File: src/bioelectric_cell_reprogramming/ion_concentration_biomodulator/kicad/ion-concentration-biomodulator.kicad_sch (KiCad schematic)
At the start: 43 parts, among them J1 532610671, J10 39-53-2045, J11 Conn_01x14_Pin, J12 Conn_01x14_Pin, J13 39-53-2045, J14 39-53-2045, J15 Conn_ARM_SWD_TagConnect_TC2030, J16 IPL1-104-01-L-D-K, J17 Conn_01x02_Pin, J18 EJ508A, J19 USB_C_Receptacle_USB2.0_14P, J2 532610671, J21 IPL1-102-01-L-S-K, J22 IPL1-104-01-X-S-K, J3 532610671, J4 532610671, J5 S4B-PH-SM4-TB, J6 Conn_01x02_Pin, J8 39-53-2045, J9 IPL1-102-01-L-S-K, Q1 NDT3055L, Q2 NDT3055L, Q4 NDT3055L, Q5 NDT3055L, Q6 NDT3055L, SW1 SW_Push, U2 LM1084-5.0, U3 LM1084-3.3, U4 USBLC6-2SC6

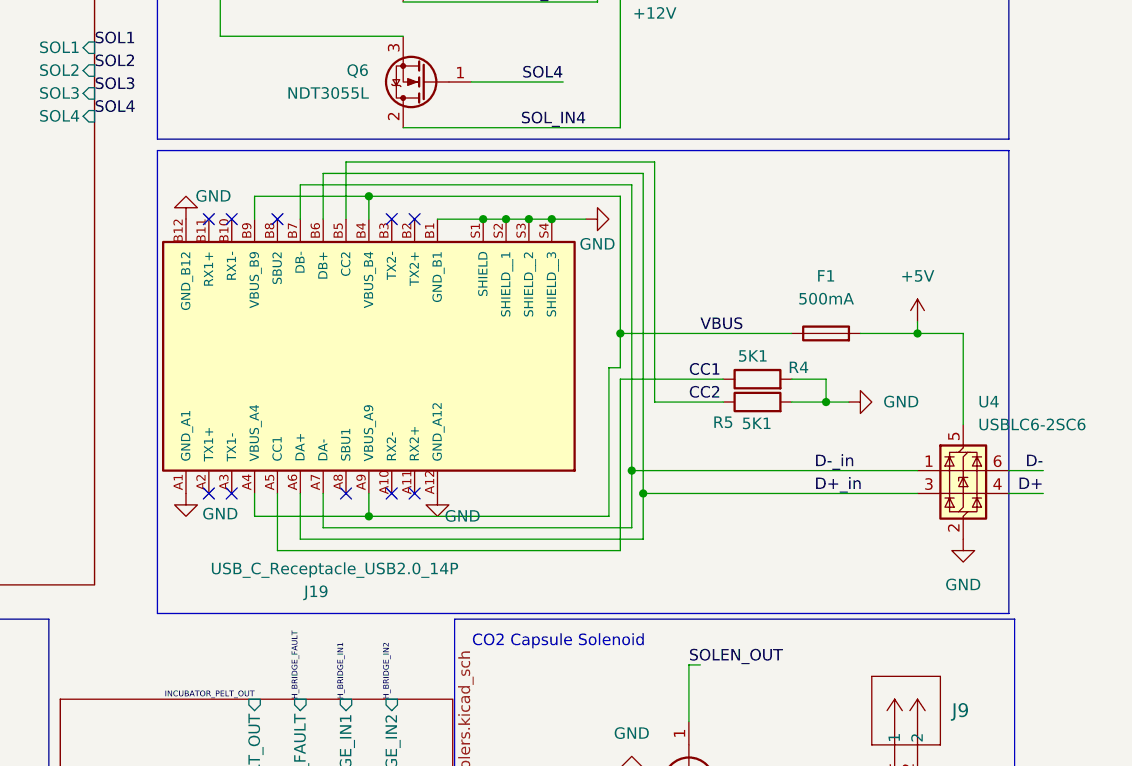
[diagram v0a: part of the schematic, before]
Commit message: feat: oscillator plus mfg files
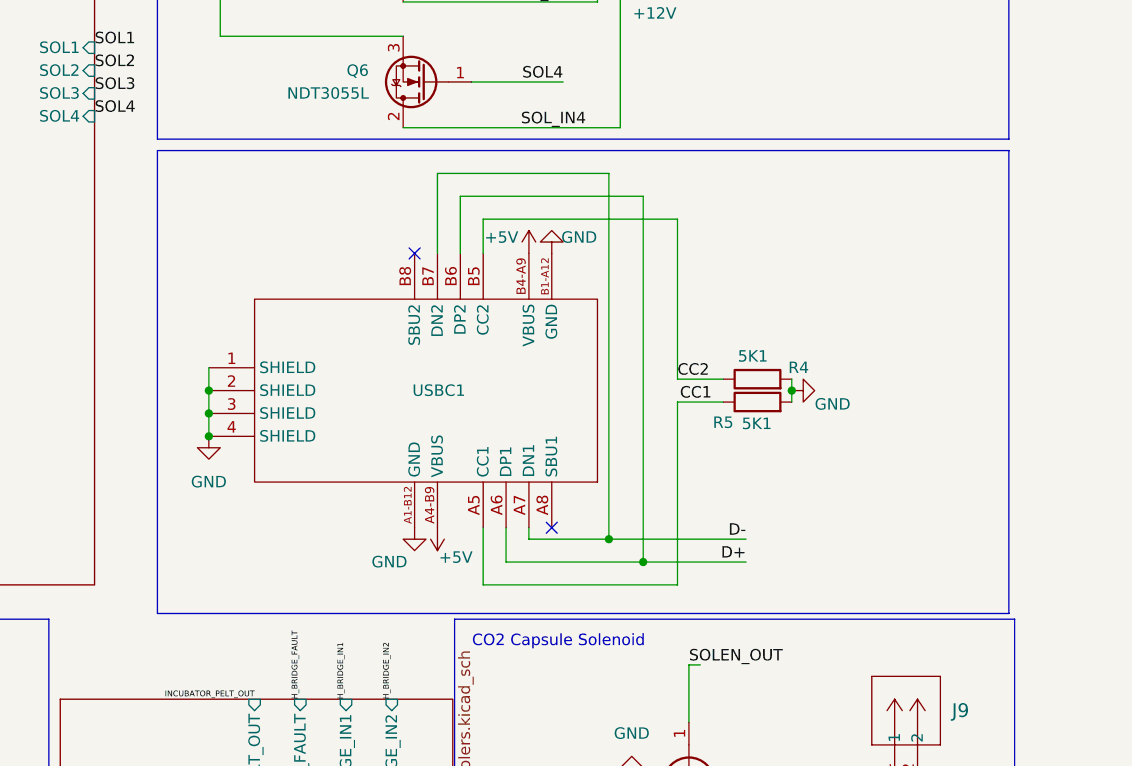
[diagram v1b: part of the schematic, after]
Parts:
- removed F1: 500mA, Fuse:Fuse_0603_1608Metric, symbol Device:Fuse
- removed J19: USB_C_Receptacle_USB2.0_14P, 12401610E4_2A.pretty:AMPHENOL_12401610E4_2A, symbol 12401610E4_2A:12401610E4_2A
- removed U4: USBLC6-2SC6, Package_TO_SOT_SMD:SOT-23-6, symbol Power_Protection:USBLC6-2SC6
- added USBC1: ~, USB-C-SMD_MC-311D:USB-C-SMD_MC-311D, symbol USB-C-SMD_MC-311D:MC-311D
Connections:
- net +5V: now also USBC1.A4-B9 (VBUS), USBC1.B4-A9 (VBUS)
- net CC1: now also R5.1, USBC1.A5 (CC1); no longer R4.1
- net CC2: now also R4.1, USBC1.B5 (CC2); no longer R5.1
- net D+: now also USBC1.A6 (DP1), USBC1.B6 (DP2)
- net D-: now also USBC1.A7 (DN1), USBC1.B7 (DN2)
- net GND: now also USBC1.1 (SHIELD), USBC1.2 (SHIELD), USBC1.3 (SHIELD), USBC1.4 (SHIELD), USBC1.A1-B12 (GND), USBC1.B1-A12 (GND)
- no-connect marks 18 -> 10
